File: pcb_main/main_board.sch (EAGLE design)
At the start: 53 parts, among them Q1 FDS5680, T1 BC847, U1 STM32F411RET6, X1 FH12-14S-0.5SH

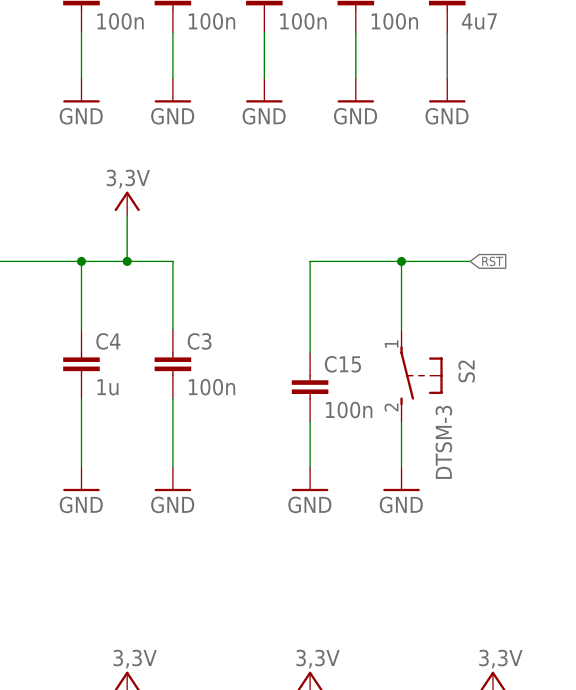
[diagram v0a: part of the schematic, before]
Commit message: before 2 H-bridges
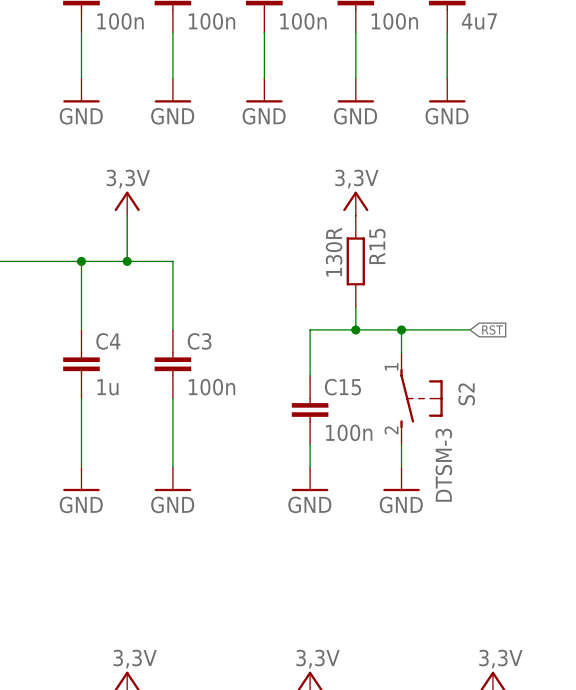
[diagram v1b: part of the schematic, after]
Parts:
- added R15: 130R, rcl:R-EU_R0603
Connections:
- net 3,3V: now also R15.1
- net RST: now also R15.2
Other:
- moved on the sheet: C15, S2
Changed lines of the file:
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@@
 <part name="GND33" library="supply1" library_urn="urn:adsk.eagle:library:371" deviceset="GND" device=""/>
 <part name="GND34" library="supply1" library_urn="urn:adsk.eagle:library:371" deviceset="GND" device=""/>
+<part name="R15" library="rcl" library_urn="urn:adsk.eagle:library:334" deviceset="R-EU_" device="R0603" package3d_urn="urn:adsk.eagle:package:23555/3" value="130R"/>
+<part name="P+1" library="supply1" library_urn="urn:adsk.eagle:library:371" deviceset="VCC" device=""/>
 </parts>
 <sheets>
@@
 </instance>
 <instance part="P+24" gate="VCC" x="10.16" y="-116.84" smashed="yes"/>
-<instance part="S2" gate="G$1" x="101.6" y="17.78" smashed="yes" rot="R180">
-<attribute name="NAME" x="107.95" y="19.685" size="1.778" layer="95" rot="R270"/>
-<attribute name="VALUE" x="105.41" y="14.605" size="1.778" layer="96" rot="R270"/>
-</instance>
-<instance part="C15" gate="G$1" x="91.44" y="17.78" smashed="yes">
-<attribute name="NAME" x="92.964" y="18.161" size="1.778" layer="95"/>
-<attribute name="VALUE" x="92.964" y="13.081" size="1.778" layer="96"/>
+<instance part="S2" gate="G$1" x="101.6" y="15.24" smashed="yes" rot="R180">
+<attribute name="NAME" x="107.95" y="17.145" size="1.778" layer="95" rot="R270"/>
+<attribute name="VALUE" x="105.41" y="12.065" size="1.778" layer="96" rot="R270"/>
+</instance>
+<instance part="C15" gate="G$1" x="91.44" y="15.24" smashed="yes">
+<attribute name="NAME" x="92.964" y="15.621" size="1.778" layer="95"/>
+<attribute name="VALUE" x="92.964" y="10.541" size="1.778" layer="96"/>
 </instance>
 <instance part="GND33" gate="1" x="91.44" y="5.08" smashed="yes">
@@
 <attribute name="VALUE" x="99.06" y="2.54" size="1.778" layer="96"/>
 </instance>
+<instance part="R15" gate="G$1" x="96.52" y="30.48" smashed="yes" rot="R270">
+<attribute name="NAME" x="98.0186" y="34.29" size="1.778" layer="95" rot="R270"/>
+<attribute name="VALUE" x="93.218" y="34.29" size="1.778" layer="96" rot="R270"/>
+</instance>
+<instance part="P+1" gate="VCC" x="96.52" y="38.1" smashed="yes"/>
 </instances>
 <busses>
@@
 <pinref part="C15" gate="G$1" pin="2"/>
 <pinref part="GND33" gate="1" pin="GND"/>
-<wire x1="91.44" y1="12.7" x2="91.44" y2="7.62" width="0.1524" layer="91"/>
+<wire x1="91.44" y1="10.16" x2="91.44" y2="7.62" width="0.1524" layer="91"/>
 </segment>
 <segment>
 <pinref part="GND34" gate="1" pin="GND"/>
 <pinref part="S2" gate="G$1" pin="2"/>
-<wire x1="101.6" y1="7.62" x2="101.6" y2="12.7" width="0.1524" layer="91"/>
+<wire x1="101.6" y1="7.62" x2="101.6" y2="10.16" width="0.1524" layer="91"/>
 </segment>
 </net>
@@
 <label x="73.66" y="40.64" size="1.778" layer="95" rot="R180"/>
 </segment>
+<segment>
+<pinref part="R15" gate="G$1" pin="1"/>
+<pinref part="P+1" gate="VCC" pin="VCC"/>
+<label x="99.06" y="40.64" size="1.778" layer="95" rot="R180"/>
+</segment>
 </net>
 <net name="BO1" class="0">
@@
 <segment>
 <pinref part="S2" gate="G$1" pin="1"/>
-<wire x1="101.6" y1="22.86" x2="101.6" y2="30.48" width="0.1524" layer="91"/>
+<wire x1="101.6" y1="20.32" x2="101.6" y2="22.86" width="0.1524" layer="91"/>
 <pinref part="C15" gate="G$1" pin="1"/>
-<wire x1="101.6" y1="30.48" x2="91.44" y2="30.48" width="0.1524" layer="91"/>
-<wire x1="91.44" y1="30.48" x2="91.44" y2="20.32" width="0.1524" layer="91"/>
-<wire x1="101.6" y1="30.48" x2="109.22" y2="30.48" width="0.1524" layer="91"/>
-<junction x="101.6" y="30.48"/>
-<label x="109.22" y="30.48" size="1.016" layer="95" xref="yes"/>
-</segment>
-</net>
+<wire x1="101.6" y1="22.86" x2="96.52" y2="22.86" width="0.1524" layer="91"/>
+<wire x1="96.52" y1="22.86" x2="91.44" y2="22.86" width="0.1524" layer="91"/>
+<wire x1="91.44" y1="22.86" x2="91.44" y2="17.78" width="0.1524" layer="91"/>
+<wire x1="101.6" y1="22.86" x2="109.22" y2="22.86" width="0.1524" layer="91"/>
+<junction x="101.6" y="22.86"/>
+<label x="109.22" y="22.86" size="1.016" layer="95" xref="yes"/>
+<pinref part="R15" gate="G$1" pin="2"/>
+<wire x1="96.52" y1="25.4" x2="96.52" y2="22.86" width="0.1524" layer="91"/>
+<junction x="96.52" y="22.86"/>
+</segment>
+</net>
